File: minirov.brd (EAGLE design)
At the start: 50.8 x 50.8 mm, 69 parts, among them Q1 DMN6140L-13DICT-ND, Q2 DMN6140L-13DICT-ND, U1 DRV8848PWP, U2 DRV8848PWP, Y1 ECS-80-S-4X

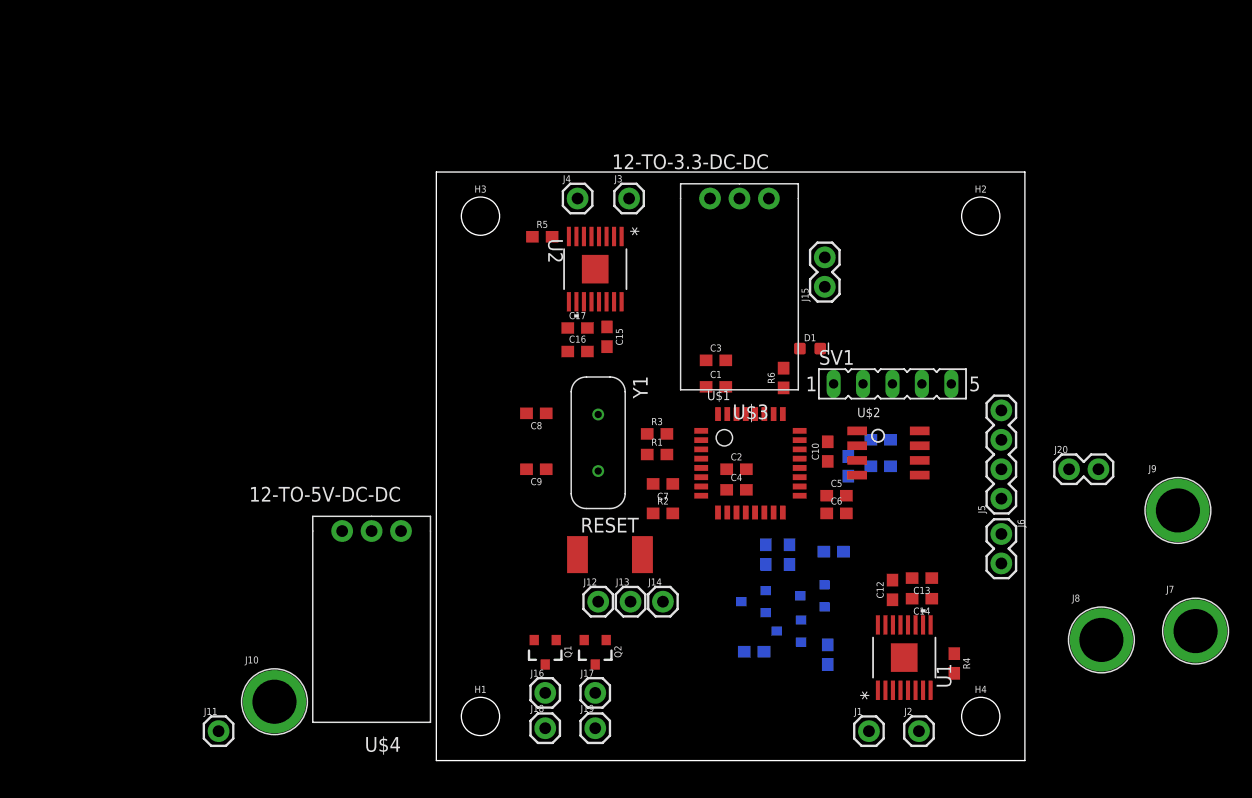
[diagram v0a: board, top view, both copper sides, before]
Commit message: first iteration of schematic and board placements
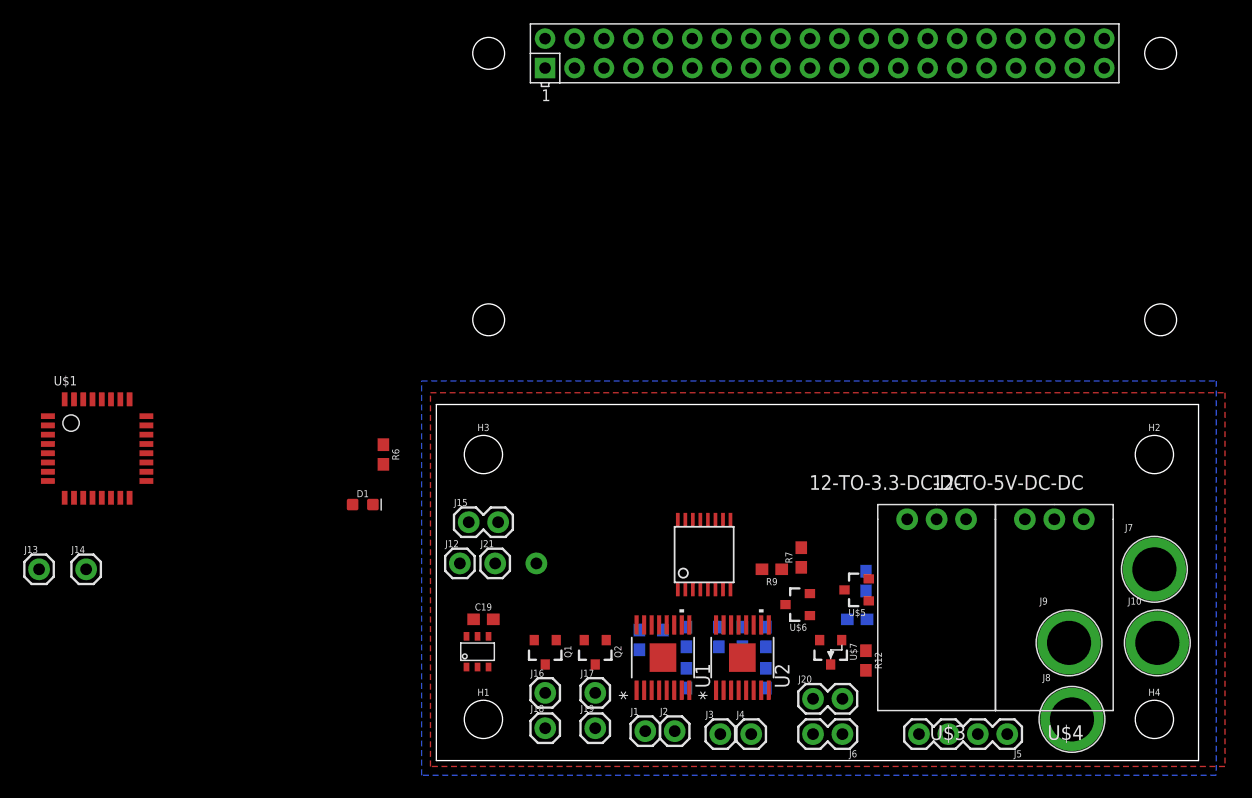
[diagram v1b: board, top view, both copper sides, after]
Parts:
- removed C1, C10, C2, C3, C4, C5, C6, C7, C8, C9: 4.7uF, SparkFun-Capacitors:0603
- removed C11: 0.1uF, SparkFun-Capacitors:0603
- removed R1, R10, R11, R2, R3: 1k, SparkFun-Resistors:0603
- removed RESET: (no value), DiscreteComponents:SW_2512
- removed SV1: (no value), con-lsta:FE05-1
- removed Y1: ECS-80-S-4X, ECS-80-S-4X:XTAL_ECS-80-S-4X
- added C19: 100nF, SparkFun-Capacitors:0603
- added J21: (no value), SparkFun-Connectors:1X01
- added U$8: TLE493DW2B6, TLE493DW2B6:TLE493DW2B6
- added U$9: RPI-ZERO, RPI-Zero:RASPBERRYPI_BASTELSTUBE_V13_RASPI_BOARD_B+_FULL
- U$2: value TCAN337D -> 74CBTLV3257PW; device PI_Shield_Library:TCAN337D -> 74CBTLV3257PW:74CBTLV3257PW
- moved J10 76.4 mm to (62.2, 10.2)
- moved U$4 58.9 mm to (53.3, 20.8)
- moved U$1 56.4 mm to (-33.5, 24.1)
- moved J13 51.1 mm to (-34.3, 16.5)
- moved J14 49.9 mm to (-30.2, 16.5)
- moved J4 48.6 mm to (27.2, 2.29)
- moved J3 46.9 mm to (24.5, 2.29)
- moved R5 42.7 mm to (28.4, 7.11), flipped to the bottom, turned to 270 degrees
- moved D1 40.9 mm to (-6.35, 22.1)
- moved J15 36.8 mm to (2.79, 20.6), turned to 0 degrees
- moved U2 35.9 mm to (26.4, 8.89), turned to 90 degrees
- moved R6 35.2 mm to (-4.57, 26.4), turned to 270 degrees
- moved U$3 32.5 mm to (43.2, 20.8)
- moved C17 31.2 mm to (28.4, 10.7), flipped to the bottom, turned to 90 degrees
- moved J11 31.0 mm to (8.64, 17.0), flipped to the bottom
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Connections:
- removed net N$3: C11.2, R10.1, R11.2
- removed net NRST: C7.1, R2.1, RESET.2, SV1.2, U$1.NRST
- removed net PWM3: U2.16
- removed net PWM4: U2.15
- new net MTR1_PWM: U$2.1A, U$9.33
- new net MTR2_PWM: U$2.2A, U$9.12
- new net MTR_AB_SEL: U$2.S, U$9.16
- new net MTR_NOE: U$2.NOE, U$9.15
- net +3V3: now also C19.2, J21.1, U$2.3V3, U$8.3V3; no longer C1.1, C10.1, C2.1, C3.1, C4.1, C5.1, C6.1, R2.2, SV1.5, U$1.VDD, U$1.VDDA, U$1.VDDIO2, U$2.VCC
- net +5V: now also U$9.2, U$9.4
- net CAN_H: no longer R10.2, U$2.CANH
- net CAN_L: no longer R11.1, U$2.CANL
- net CAN_STM_RX: no longer U$2.TXD
- net CAN_STM_TX: no longer U$2.RXD
- net GND: now also C19.1, U$8.GND1, U$8.GND2, U$8.GND3, U$9.14, U$9.20, U$9.25, U$9.30, U$9.34, U$9.39, U$9.6, U$9.9; no longer C1.2, C10.2, C11.1, C2.2, C3.2, C4.2, C5.2, C6.2, C7.2, C8.2, C9.2, RESET.1, SV1.1
- net LED1_PWM: now also U$9.11; no longer U$1.PA6
- net LED2_PWM: now also U$9.13; no longer U$1.PA7
- net MISO: now also U$9.21; no longer U$1.PB4
- net MOSI: now also U$9.19; no longer U$1.PB5
- net MTR_1A_PWM: now also U$2.1B1; no longer U$1.PA0
- net MTR_1B_PWM: now also U$2.1B2; no longer U$1.PA1
- net MTR_2A_PWM: now also U$2.2B1, U2.16; no longer U$1.PA2
- net MTR_2B_PWM: now also U$2.2B2, U2.15; no longer U$1.PA3
- net N$1: now also U$9.8; no longer C9.1, R1.1, Y1.2
- net N$2: now also U$9.10; no longer C8.1, R3.1, Y1.1
- net OSC_IN: no longer R3.2
- net OSC_OUT: no longer R1.2
- net SCK: now also U$9.23; no longer U$1.PB3
- net SCL: now also U$8.SCL, U$9.5; no longer U$1.PB6
- net SDA: now also U$8.SDA, U$9.3; no longer U$1.PB7
- net SWCLK: no longer SV1.3
- net SWDIO: no longer SV1.4
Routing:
- added copper zone on layer 1, net GND
- added copper zone on layer 16, net GND
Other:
- board size 50.8 x 50.8 mm -> 65.8 x 30.7 mm
